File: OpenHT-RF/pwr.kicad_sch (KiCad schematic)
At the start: 54 parts, among them J201 Conn_01x02, SW201 436351045816, U201 LTC2954-1, U202 TPS65261RHBx, U203 AP7330-W5-7

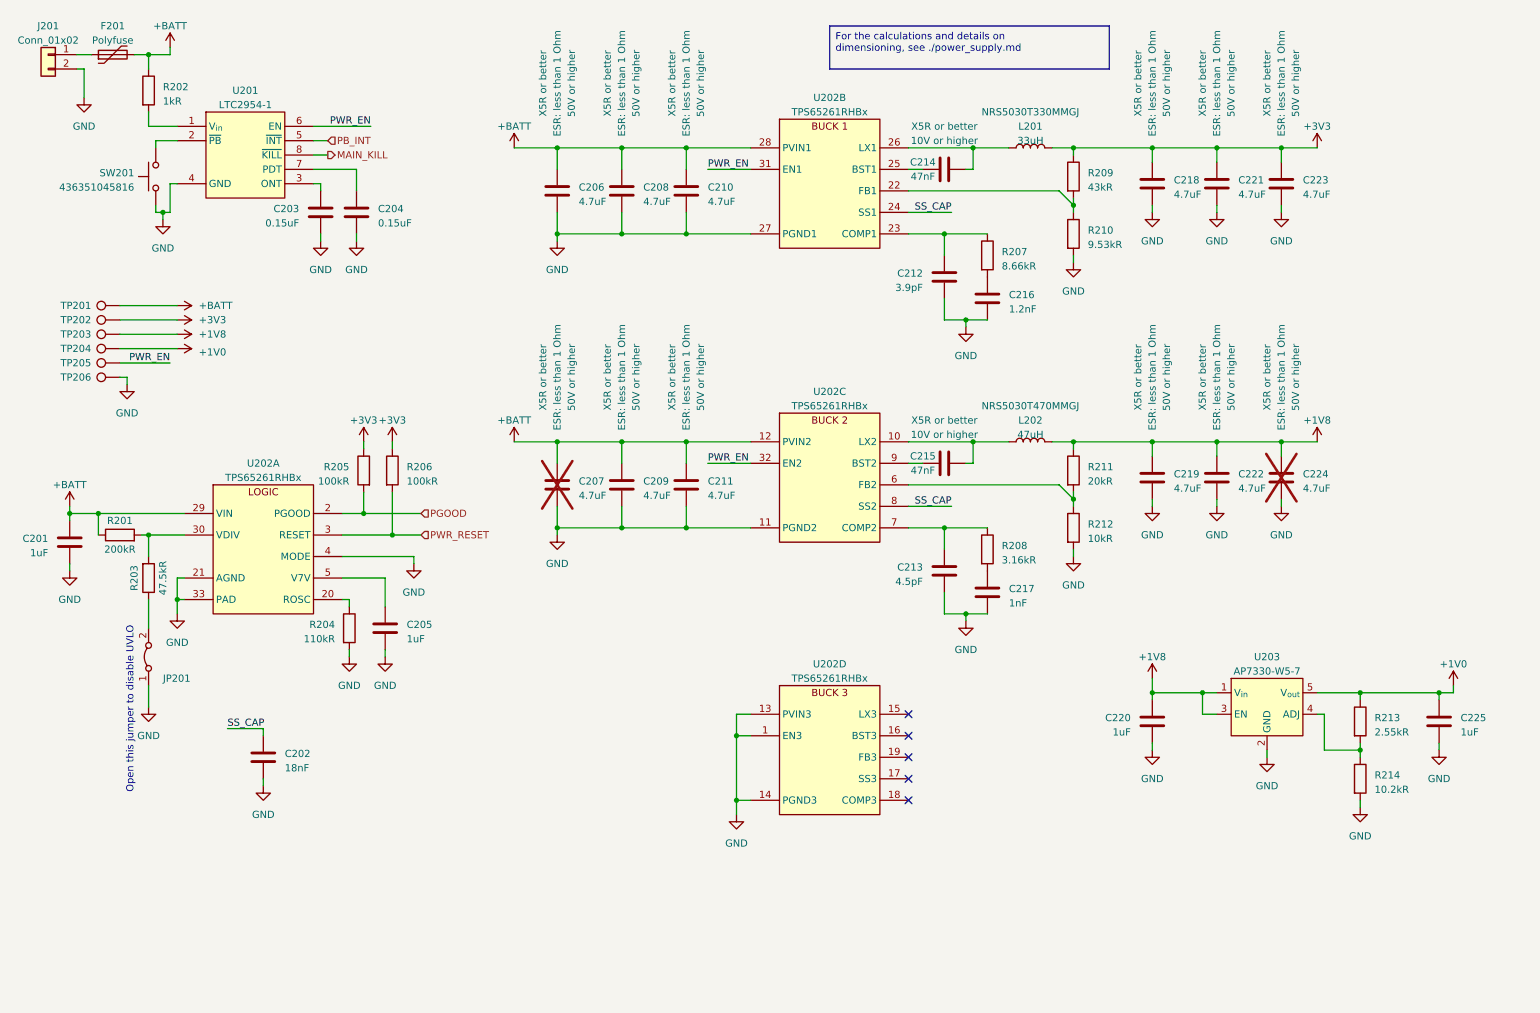
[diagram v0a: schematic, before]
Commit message: Added a load switch for the nucleo board
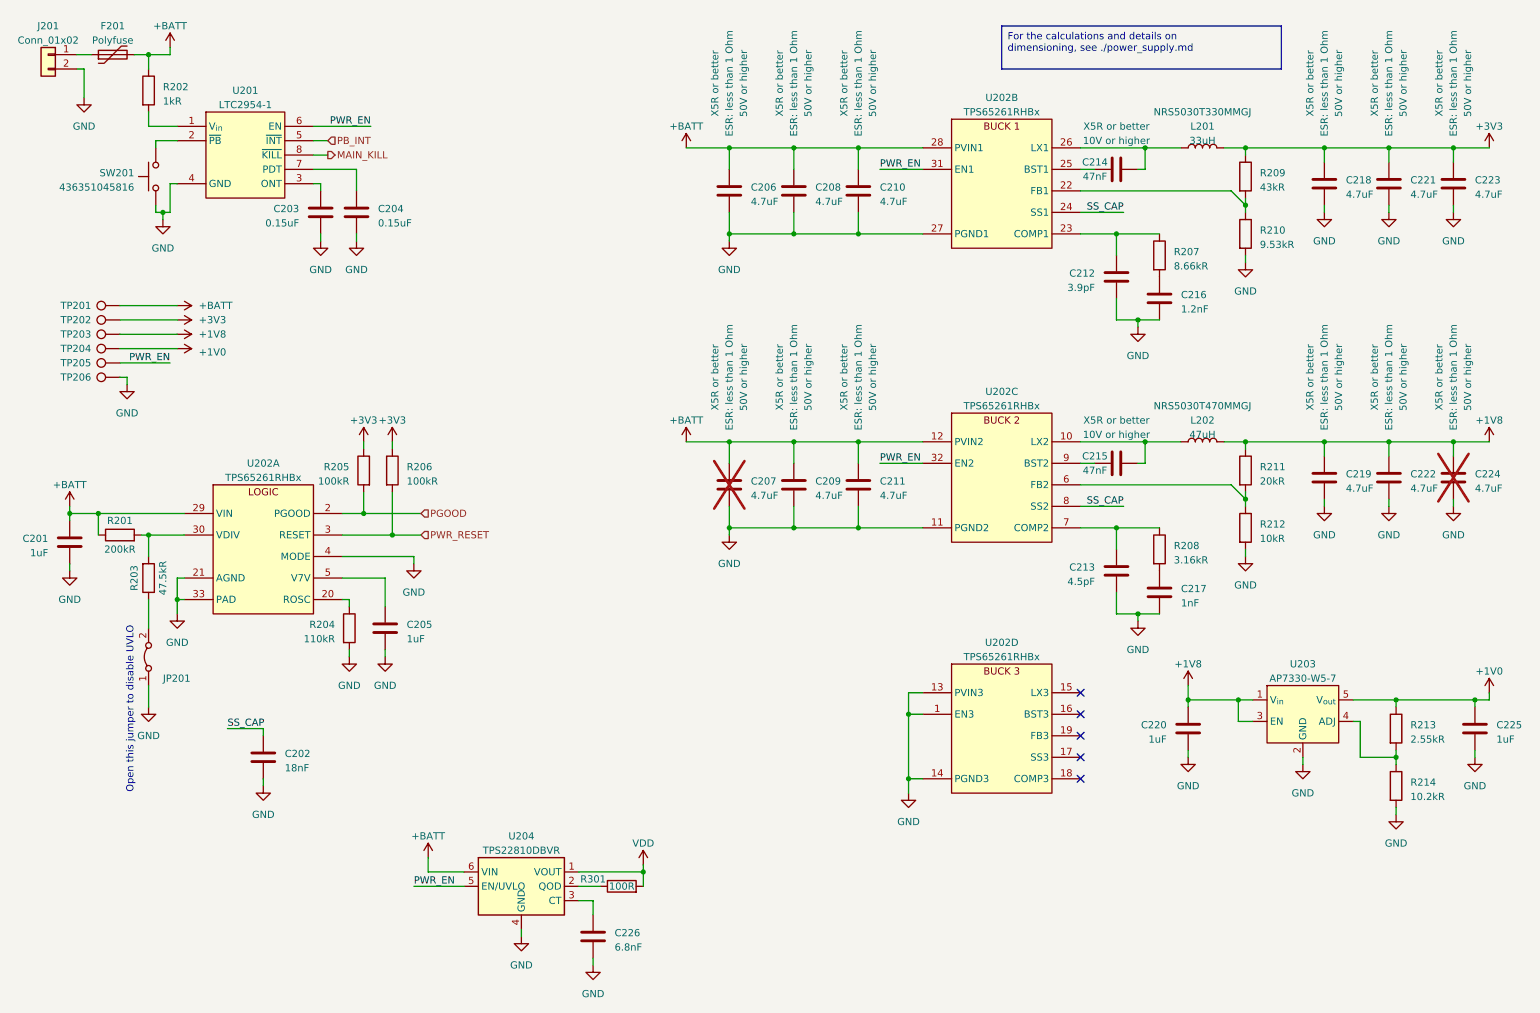
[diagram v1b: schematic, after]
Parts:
- added C226: 6.8nF, Capacitor_SMD:C_0402_1005Metric, symbol Device:C
- added R301: 100R, Resistor_SMD:R_0402_1005Metric, symbol Device:R
- added U204: TPS22810DBVR, Package_TO_SOT_SMD:SOT-23-6, symbol Power_Management:TPS22810DRV
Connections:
- net +BATT: now also U204.6 (VIN)
- net GND: now also C226.2, U204.4 (GND), U204.7 (GND)
- net PWR_EN: now also U204.5 (EN/UVLO)
- new net: R301.1, U204.2 (QOD)
- new net: C226.1, U204.3 (CT)
- new net VDD: R301.2, U204.1 (VOUT)
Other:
- moved on the sheet: C206, C207, C208, C209, C210, C211, C212, C213, C214, C215, C216, C217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
